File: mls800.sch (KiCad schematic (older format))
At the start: 47 parts, among them CON1 BARREL_JACK, IC1 6N137, J1 USB, P1 CONN_02X03, P2 DIN_5, P3 DIN_5, P4 CONN_02X03, P5 CONN_02X03, SW12 SW_PUSH, U1 LM340MP-5.0/NOPB, U2 ATmega32U4-AU, U3 24LC256, X1 16Mhz

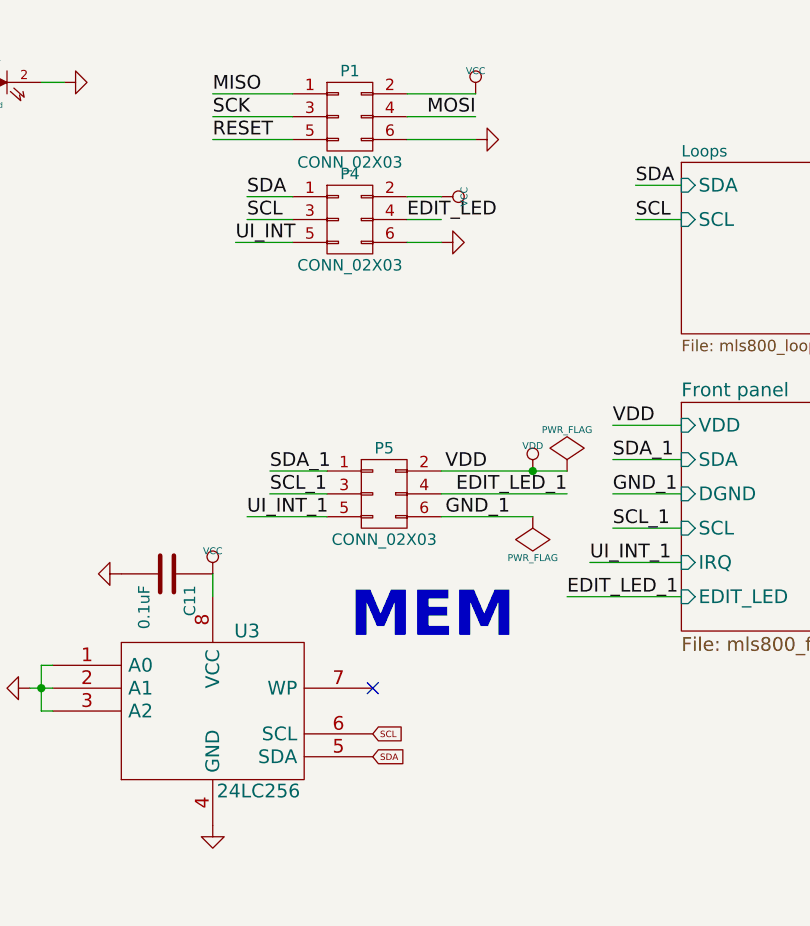
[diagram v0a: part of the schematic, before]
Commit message: MLS800
* copper zone clearance
* round drilling holes
*
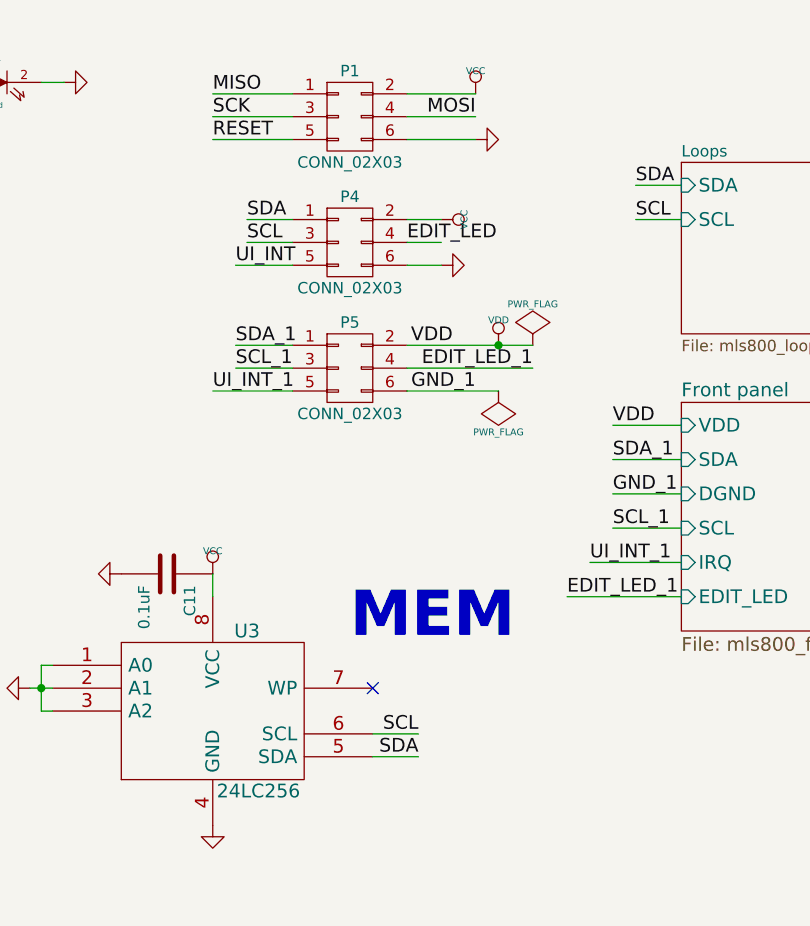
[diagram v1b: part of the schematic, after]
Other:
- moved on the sheet: P4, P5
